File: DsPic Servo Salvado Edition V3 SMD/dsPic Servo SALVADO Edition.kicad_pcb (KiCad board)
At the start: 2 copper layers, 48.3 x 49.5 mm, 37 parts, among them Con3 24 V, Con4 HEIDELBERG_4, Con5 RC15, Con6 PicKit IF, Con7 MOTOR, IC2 dsPIC30F4012, IC3 LM2904, IC4 L6203, J1 Prog

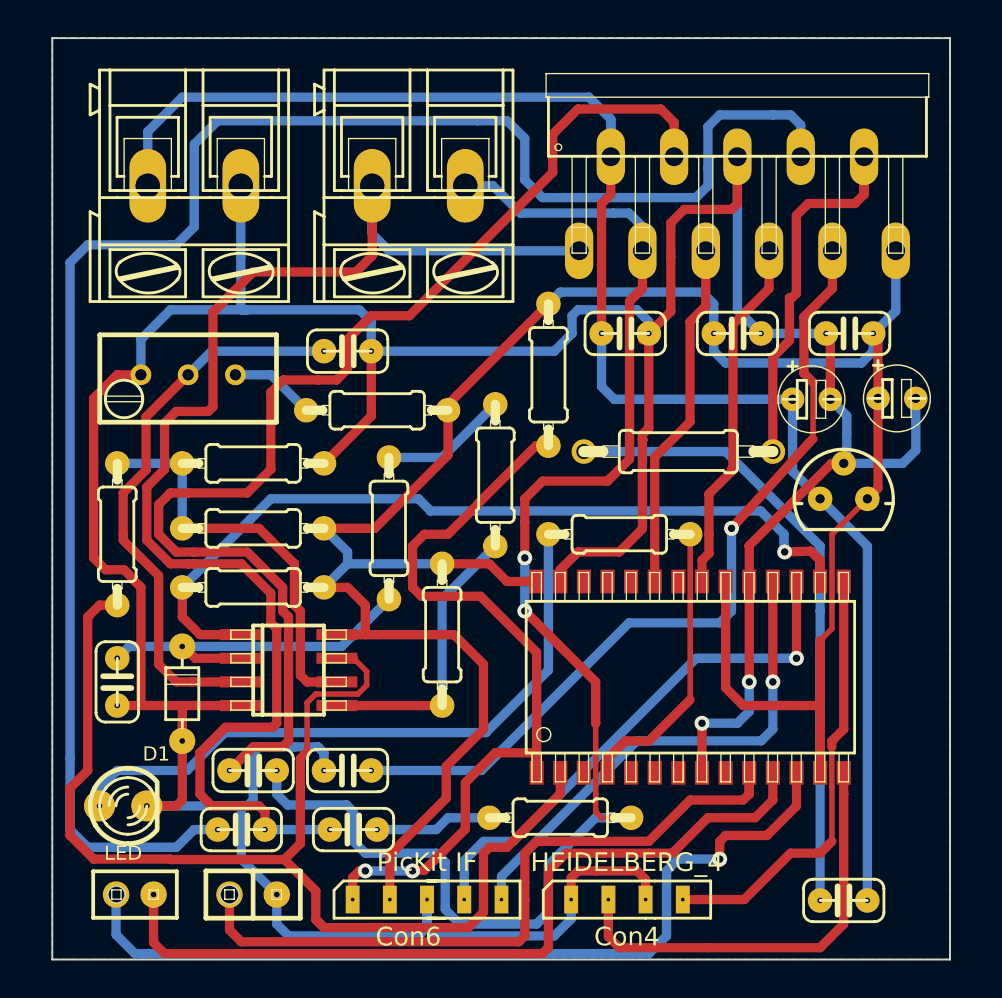
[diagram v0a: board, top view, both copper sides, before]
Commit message: Add files via upload
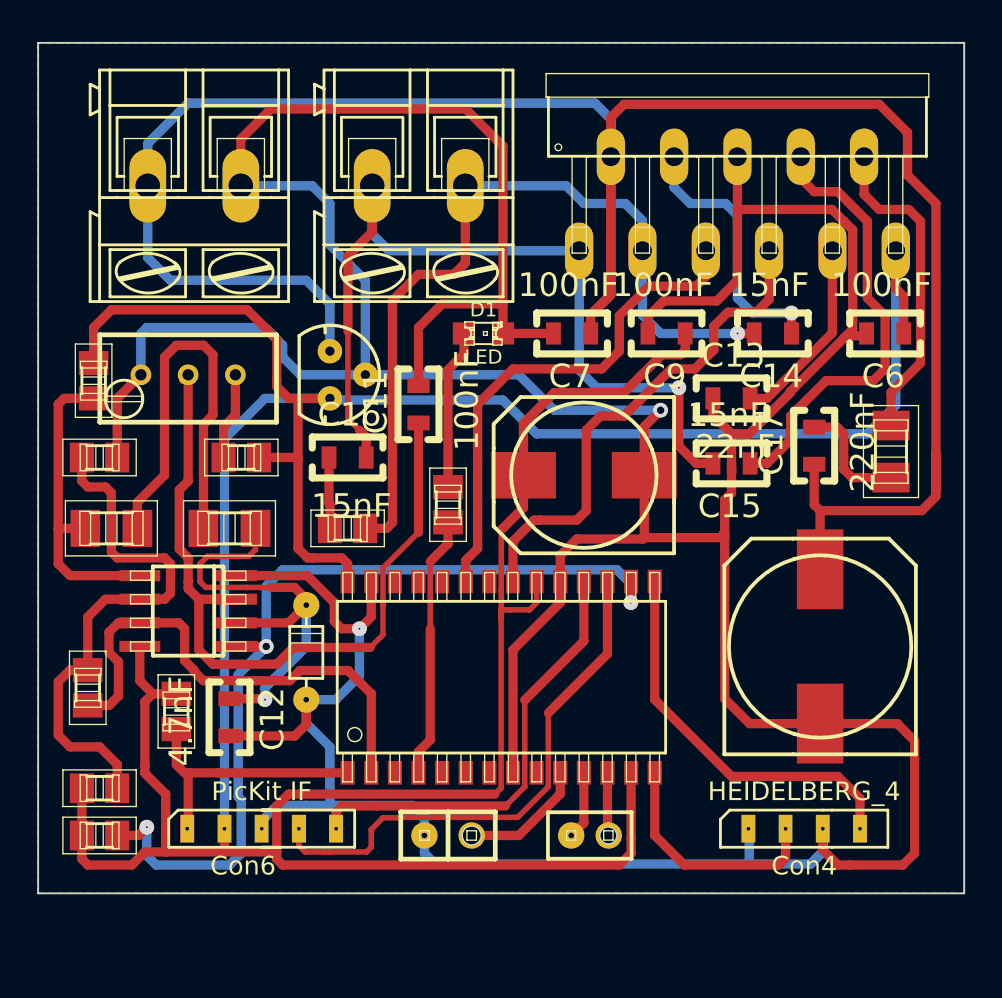
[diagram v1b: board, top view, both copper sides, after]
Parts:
- C10: footprint Cap-Pol-TH:CAP-POL-TH-E2-5 -> Cap-Pol-SMD:140CLH-0810
- C11, C12, C13, C14, C15, C16, C17, C6, C7, C9: footprint Cap-TH:CAP-TH-C025-024X044 -> Cap-SMD:CAP-SMD-0805
- C8: footprint Cap-Pol-TH:CAP-POL-TH-E2-5 -> Cap-Pol-SMD:140CLH-1010
- D1: footprint Led:LED-3MM -> Led:LED-0805
- R10, R12, R13, R14, R15, R16, R5, R6, R7: footprint Resistors-TH:RES-TH-0204_7 -> Resistors-SMD:M0805
- R11, R9: footprint Resistors-TH:RES-TH-0204_7 -> Resistors-SMD:M1206
- RSense1: footprint Resistors-TH:RES-TH-0207_10 -> Resistors-SMD:M1206
- moved C14 36.5 mm to (92.1, 56.5), turned to 180 degrees
- moved C15 32.9 mm to (89.9, 63.5), turned to 180 degrees
- moved D1 31.9 mm to (76.5, 56.5)
- moved C13 28.7 mm to (89.9, 60.0)
- moved Reg1 28.4 mm to (68.3, 58.7), turned to 270 degrees
- moved R6 27.0 mm to (60.0, 76.8)
- moved J1 24.7 mm to (82.2, 83.5), turned to 180 degrees
- moved C17 24.5 mm to (94.3, 62.5), turned to 90 degrees
- moved R13 23.2 mm to (55.6, 59.1)
- moved R11 20.8 mm to (56.5, 67.0), turned to 0 degrees
- moved C16 20.0 mm to (69.2, 63.2), turned to 0 degrees
- moved R16 19.3 mm to (69.2, 67.0)
- moved C10 17.3 mm to (81.9, 64.1), turned to 180 degrees
- moved R12 16.2 mm to (55.9, 81.0), turned to 180 degrees
- moved R10 15.7 mm to (55.9, 83.5), turned to 0 degrees
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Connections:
- IC2 pad 22: (no net) -> PWM_L_B
- IC2 pad 24: (no net) -> PWM_L_A
- IC2 pad 25: (no net) -> Net-(IC2-Pad25)
- IC2 pad 26: (no net) -> Net-(IC2-Pad26)
- IC2 pad 3: (no net) -> ENABLE
- IC2 pad 5: (no net) -> INDX
- IC2 pad 6: (no net) -> QEA
- IC2 pad 7: (no net) -> QEB
- IC2 pad 9: (no net) -> Net-(IC2-Pad9)
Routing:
- net +5V: track 124.2 -> 208.3 mm
- net Net-(C15-Pad1): track 95.5 -> 24.1 mm
- net GND: track 212.8 -> 268.1 mm
- net Net-(C14-Pad1): track 64.9 -> 14.5 mm, vias 0 -> 1
- net Net-(IC2-Pad12): track 47.0 -> 3.40 mm, vias 1 -> 0
- net Net-(IC2-Pad11): track 43.4 -> 3.65 mm
- net +24V: track 84.8 -> 122.9 mm
- net /CPU/AN0: track 65.1 -> 27.1 mm
- net Net-(C14-Pad2): track 81.3 -> 45.8 mm, vias 2 -> 1
- net Net-(C13-Pad2): track 44.8 -> 10.3 mm, vias 1 -> 0
- net /CPU/RC15: track 38.3 -> 6.82 mm
- net Net-(C17-Pad2): track 33.9 -> 6.37 mm
- net MCLR: track 41.7 -> 14.4 mm, vias 2 -> 0
- net Net-(D1-Pad1): track 35.0 -> 8.61 mm
- net Net-(C15-Pad2): track 72.8 -> 47.2 mm, vias 0 -> 1
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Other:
- board size 48.3 x 49.5 mm -> 49.8 x 45.7 mm
- net class 04: via_drill 0.4 -> 0.1
- net class Default: via_drill 0.4 -> 0.1
- net class Power: via_dia 0.8 -> 4; via_drill 0.4 -> 0.1
- rule via_min_drill: 0.3 -> 0.1
